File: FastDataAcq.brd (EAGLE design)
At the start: 114.3 x 63.2 mm, 223 parts, among them IC1 LT1963AEQ, IC2 FT230XQ, IC3 ADCMP553BRMZ, J1 MICRO-FIT_3.0_2POS_RA_SMD, J2 USB_MICROAB_SMT, J3 HEADER_0.1"_10P_2R_SMT, X1 87832-14, X2 SMA-142-0701-801/806, X3 SMA-142-0701-801/806, Y1 SI530-500, Y2 100MHz, Y3 DNP

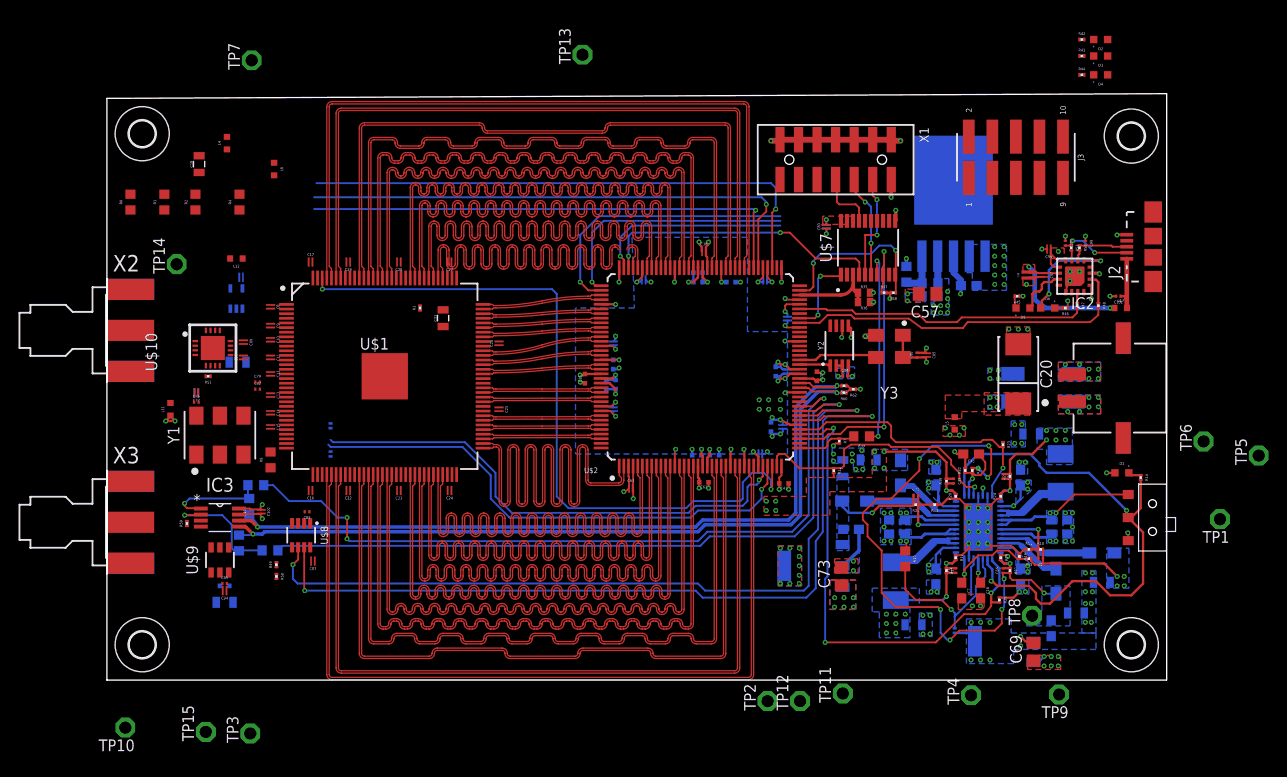
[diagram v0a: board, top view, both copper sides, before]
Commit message: Digital layout complete.
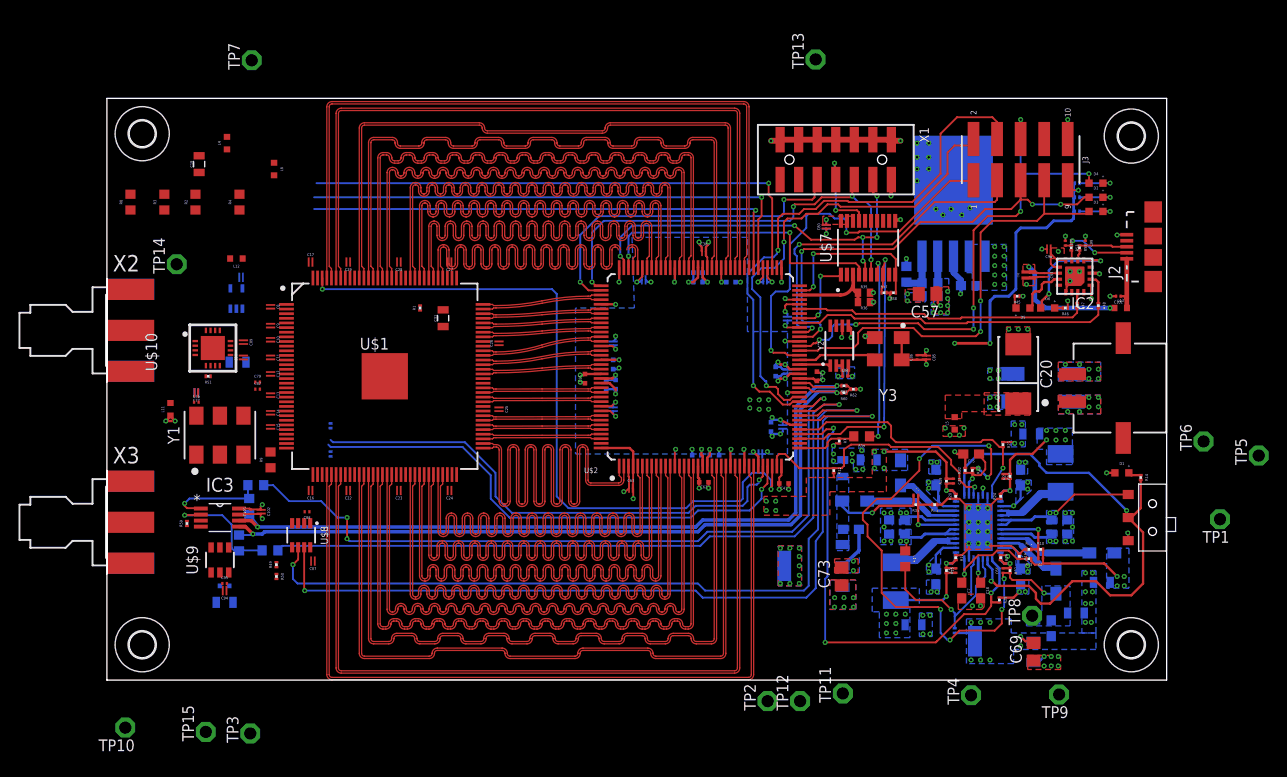
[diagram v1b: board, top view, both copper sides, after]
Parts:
- moved TP13 25.2 mm to (76.4, 84.2)
- moved D2 17.0 mm to (106.7, 69.3), turned to 0 degrees
- moved R42 17.0 mm to (104.6, 69.3), flipped to the bottom, turned to 180 degrees
- moved D3 16.8 mm to (106.7, 67.8), turned to 0 degrees
- moved R43 16.8 mm to (104.6, 67.8), flipped to the bottom, turned to 180 degrees
- moved D4 11.7 mm to (106.7, 70.9), turned to 0 degrees
- moved R44 11.7 mm to (104.6, 70.9), flipped to the bottom, turned to 180 degrees
- moved J3 0.57 mm to (98.6, 73.4)
- moved Y3 0.28 mm to (84.3, 53.0)
- moved C85 0.25 mm to (88.4, 52.1)
- moved C86 0.25 mm to (87.4, 52.1)
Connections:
- removed net N3: U$2.P$62
- removed net N4: U$2.P$61
- removed net N5: U$2.P$59
- removed net N6: U$2.P$58
- removed net N7: U$2.P$57
- removed net N8: U$2.P$48
- removed net N9: U$2.P$47
- net 3V3: now also J3.P$9; no longer J3.P$1
- net FPGA_GPIO1: now also J3.P$4, U$2.P$47; no longer J3.P$9
- net FPGA_GPIO2: now also J3.P$2, U$2.P$48; no longer J3.P$8
- net FPGA_GPIO3: now also J3.P$1, U$2.P$57; no longer J3.P$7
- net FPGA_GPIO4: now also D3.CATHODE, J3.P$7, U$2.P$58; no longer J3.P$6
- net FPGA_GPIO5: now also J3.P$6, U$2.P$59; no longer J3.P$5
- net FPGA_GPIO6: now also D2.CATHODE, J3.P$5, U$2.P$61; no longer D3.CATHODE, J3.P$4
- net FPGA_GPIO7: now also U$2.P$62; no longer D2.CATHODE
- net GND: now also J3.P$10; no longer J3.P$2
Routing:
- net FPGA_GPIO1: track 0.00 -> 59.0 mm, vias 0 -> 2
- net FPGA_GPIO5: track 0.00 -> 57.6 mm, vias 0 -> 7
- net FPGA_GPIO2: track 0.00 -> 51.6 mm, vias 0 -> 2
- net FPGA_GPIO4: track 0.00 -> 48.7 mm, vias 0 -> 2
- net FPGA_GPIO6: track 0.00 -> 48.6 mm, vias 0 -> 4
- net FPGA_GPIO3: track 0.00 -> 42.2 mm, vias 0 -> 2
- net FPGA_GPIO7: track 0.00 -> 38.0 mm, vias 0 -> 2
- net 3V3: track 51.8 -> 83.8 mm, vias 27 -> 30
- net FPGA_TCK: track 38.4 -> 49.1 mm, vias 3 -> 4
- net FPGA_TMS: track 32.9 -> 42.8 mm, vias 3 -> 6
- net FPGA_TDI: track 30.1 -> 37.8 mm, vias 1 -> 2
- net GND: track 122.2 -> 128.4 mm, vias 140 -> 151
- net 1V8: track 49.6 -> 55.5 mm
- net PROM_TDO: track 6.54 -> 10.7 mm, vias 0 -> 2
- net N$22: track 0.00 -> 4.07 mm, vias 0 -> 1
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- added copper zone on layer 1, net 1V9
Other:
- board size 114.3 x 63.2 mm -> 114.3 x 62.7 mm
